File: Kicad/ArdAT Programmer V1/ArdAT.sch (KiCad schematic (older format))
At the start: 20 parts

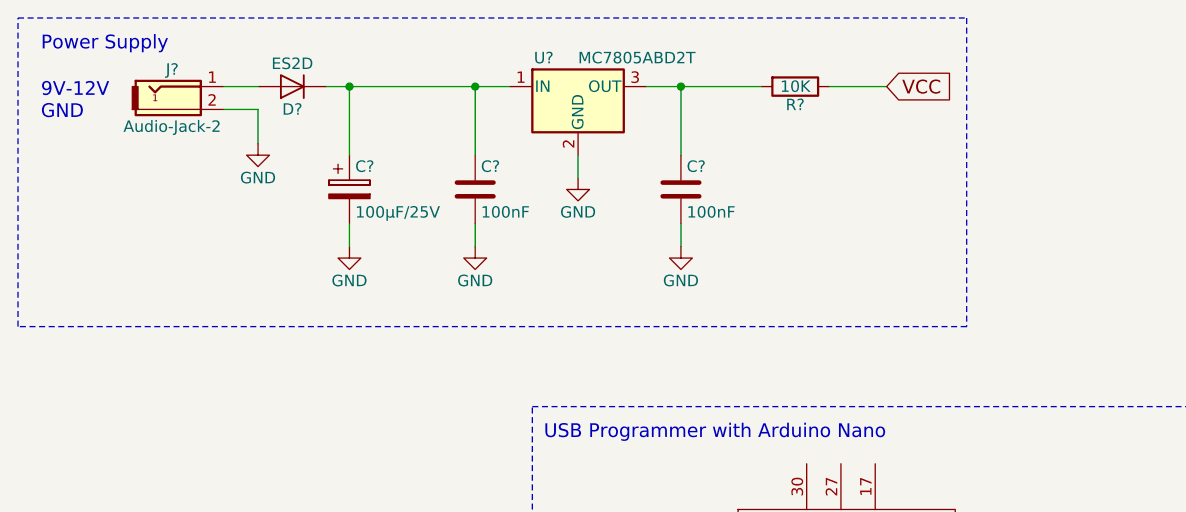
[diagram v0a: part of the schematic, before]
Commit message: Update
Update 3.3V
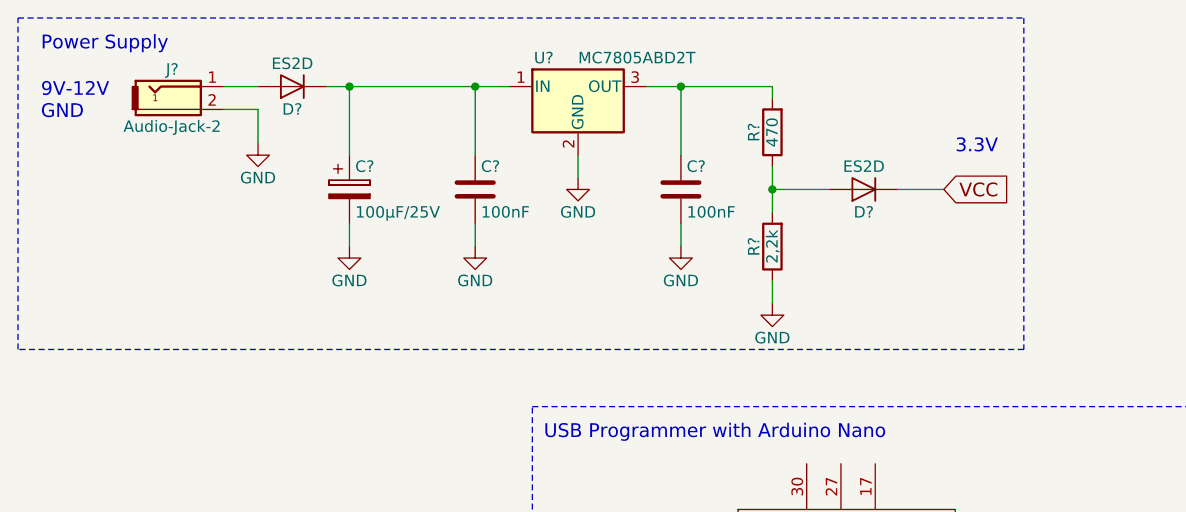
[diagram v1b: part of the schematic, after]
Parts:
- removed R?: 10K, symbol R
- added D?: ES2D, symbol D
- added R?: 470, symbol R
- added R?: 2,2k, symbol R
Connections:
- net GND: now also R?.1
- net VCC: now also D?.1 (K)
- net at C?.1, U?.3 (OUT): now also R?.2
- new net: D?.2 (A), R?.1, R?.2
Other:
- note added: "3.3V"
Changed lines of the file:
@@
 	1    0    0    -1
 $EndComp
-$Comp
-L R R?
-U 1 1 5AD70BC0
-P 4500 1000
-F 0 "R?" V 4580 1000 50  0000 C CNN
-F 1 "10K" V 4500 1000 50  0000 C CNN
-F 2 "" V 4430 1000 50  0001 C CNN
-F 3 "" H 4500 1000 50  0001 C CNN
-	1    4500 1000
-	0    1    1    0
-$EndComp
-Text GLabel 4900 1000 2    60   Input ~ 0
+Text GLabel 5150 1450 2    60   Input ~ 0
 VCC
 Text GLabel 8950 4000 0    60   Input ~ 0
@@
 F 3 "" H 2050 1000 50  0001 C CNN
 	1    1800 1000
-	1    0    0    -1
-$EndComp
-$Comp
-L MC7805ABD2T U?
-U 1 1 5AD7334E
-P 3550 1000
-F 0 "U?" H 3400 1125 50  0000 C CNN
-F 1 "MC7805ABD2T" H 3550 1125 50  0000 L CNN
-F 2 "" H 3575 850 50  0001 L CIN
-F 3 "" H 3550 950 50  0001 C CNN
-	1    3550 1000
 	1    0    0    -1
 $EndComp
@@
 	1550 6750 1550 5850
 Wire Wire Line
+	3100 1600 3100 1700
+Wire Wire Line
+	2550 1600 2550 1700
+Wire Wire Line
+	4000 1600 4000 1700
+Wire Wire Line
+	8950 3850 9400 3850
+Wire Wire Line
+	9400 3850 9400 3950
+Wire Wire Line
+	9400 3950 9500 3950
+Wire Wire Line
+	8950 4000 9350 4000
+Wire Wire Line
+	9350 4000 9350 4050
+Wire Wire Line
+	9350 4050 9500 4050
+Wire Wire Line
+	8950 4150 9500 4150
+Wire Wire Line
+	8950 4300 9350 4300
+Wire Wire Line
+	9350 4300 9350 4250
+Wire Wire Line
+	9350 4250 9500 4250
+Wire Wire Line
+	8950 4450 9400 4450
+Wire Wire Line
+	9400 4450 9400 4350
+Wire Wire Line
+	9400 4350 9500 4350
+Wire Wire Line
+	9500 4450 9450 4450
+Wire Wire Line
+	9450 4450 9450 4650
+Wire Wire Line
+	2000 1000 2150 1000
+Wire Wire Line
+	2000 1100 2150 1100
+Wire Wire Line
+	2150 1100 2150 1250
+Wire Notes Line
+	3350 2400 7300 2400
+Wire Notes Line
+	7300 2400 7300 6000
+Wire Notes Line
+	7300 6000 3350 6000
+Wire Notes Line
+	3350 6000 3350 2400
+Wire Notes Line
+	9150 5050 9450 5050
+Wire Notes Line
+	9450 5050 9450 5500
+Wire Notes Line
+	9450 5500 9150 5500
+Wire Notes Line
+	9150 5500 9150 5350
+Wire Notes Line
+	9100 5350 9450 5350
+Wire Notes Line
+	9100 5350 9100 5200
+Wire Notes Line
+	9100 5200 9450 5200
+Wire Notes Line
+	9150 5200 9150 5050
+Wire Notes Line
+	9300 5050 9300 5500
+Wire Notes Line
+	8550 3500 10350 3500
+Wire Notes Line
+	10350 3500 10350 5600
+Wire Notes Line
+	10350 5600 8550 5600
+Wire Notes Line
+	8550 5600 8550 3500
+$Comp
+L D D?
+U 1 1 5AD84211
+P 4800 1450
+F 0 "D?" H 4800 1550 50  0000 C CNN
+F 1 "ES2D" H 4800 1350 50  0000 C CNN
+F 2 "" H 4800 1450 50  0001 C CNN
+F 3 "" H 4800 1450 50  0001 C CNN
+	1    4800 1450
+	-1   0    0    1
+$EndComp
+Connection ~ 2550 1000
+Wire Wire Line
+	2550 1300 2550 1000
+Connection ~ 3100 1000
+Wire Wire Line
+	3100 1000 3100 1300
+Wire Wire Line
 	2450 1000 3250 1000
 Wire Wire Line
-	2550 1300 2550 1000
-Connection ~ 2550 1000
-Wire Wire Line
-	3100 1000 3100 1300
-Connection ~ 3100 1000
-Wire Wire Line
-	3850 1000 4350 1000
-Wire Wire Line
-	4000 1000 4000 1300
-Wire Wire Line
 	3550 1300 3550 1400
-Wire Wire Line
-	3100 1600 3100 1700
-Wire Wire Line
-	2550 1600 2550 1700
-Wire Wire Line
-	4000 1600 4000 1700
+$Comp
+L MC7805ABD2T U?
+U 1 1 5AD7334E
+P 3550 1000
+F 0 "U?" H 3400 1125 50  0000 C CNN
+F 1 "MC7805ABD2T" H 3550 1125 50  0000 L CNN
+F 2 "" H 3575 850 50  0001 L CIN
+F 3 "" H 3550 950 50  0001 C CNN
+	1    3550 1000
+	1    0    0    -1
+$EndComp
+$Comp
+L R R?
+U 1 1 5AD85C6A
+P 4400 1200
+F 0 "R?" V 4480 1200 50  0000 C CNN
+F 1 "470" V 4400 1200 50  0000 C CNN
+F 2 "" V 4330 1200 50  0001 C CNN
+F 3 "" H 4400 1200 50  0001 C CNN
+	1    4400 1200
+	-1   0    0    1
+$EndComp
+$Comp
+L R R?
+U 1 1 5AD85DF3
+P 4400 1700
+F 0 "R?" V 4480 1700 50  0000 C CNN
+F 1 "2,2k" V 4400 1700 50  0000 C CNN
+F 2 "" V 4330 1700 50  0001 C CNN
+F 3 "" H 4400 1700 50  0001 C CNN
+	1    4400 1700
+	-1   0    0    1
+$EndComp
+$Comp
+L GND #PWR?
+U 1 1 5AD85E4B
+P 4400 1950
+F 0 "#PWR?" H 4400 1700 50  0001 C CNN
+F 1 "GND" H 4400 1800 50  0000 C CNN
+F 2 "" H 4400 1950 50  0001 C CNN
+F 3 "" H 4400 1950 50  0001 C CNN
+	1    4400 1950
+	1    0    0    -1
+$EndComp
+Wire Wire Line
+	3850 1000 4400 1000
+Wire Wire Line
+	4400 1000 4400 1050
+Wire Wire Line
+	4400 1350 4400 1550
+Wire Wire Line
+	4650 1450 4400 1450
+Connection ~ 4400 1450
+Wire Wire Line
+	4000 1300 4000 1000
 Connection ~ 4000 1000
 Wire Wire Line
-	4650 1000 4900 1000
-Wire Wire Line
-	8950 3850 9400 3850
-Wire Wire Line
-	9400 3850 9400 3950
-Wire Wire Line
-	9400 3950 9500 3950
-Wire Wire Line
-	8950 4000 9350 4000
-Wire Wire Line
-	9350 4000 9350 4050
-Wire Wire Line
-	9350 4050 9500 4050
-Wire Wire Line
-	8950 4150 9500 4150
-Wire Wire Line
-	8950 4300 9350 4300
-Wire Wire Line
-	9350 4300 9350 4250
-Wire Wire Line
-	9350 4250 9500 4250
-Wire Wire Line
-	8950 4450 9400 4450
-Wire Wire Line
-	9400 4450 9400 4350
-Wire Wire Line
-	9400 4350 9500 4350
-Wire Wire Line
-	9500 4450 9450 4450
-Wire Wire Line
-	9450 4450 9450 4650
-Wire Wire Line
-	2000 1000 2150 1000
-Wire Wire Line
-	2000 1100 2150 1100
-Wire Wire Line
-	2150 1100 2150 1250
-Wire Notes Line
-	1100 700  5250 700
-Wire Notes Line
-	5250 700  5250 2050
-Wire Notes Line
-	5250 2050 1100 2050
-Wire Notes Line
-	1100 2050 1100 700
-Wire Notes Line
-	3350 2400 7300 2400
-Wire Notes Line
-	7300 2400 7300 6000
-Wire Notes Line
-	7300 6000 3350 6000
-Wire Notes Line
-	3350 6000 3350 2400
-Wire Notes Line
-	9150 5050 9450 5050
-Wire Notes Line
-	9450 5050 9450 5500
-Wire Notes Line
-	9450 5500 9150 5500
-Wire Notes Line
-	9150 5500 9150 5350
-Wire Notes Line
-	9100 5350 9450 5350
-Wire Notes Line
-	9100 5350 9100 5200
-Wire Notes Line
-	9100 5200 9450 5200
-Wire Notes Line
-	9150 5200 9150 5050
-Wire Notes Line
-	9300 5050 9300 5500
-Wire Notes Line
-	8550 3500 10350 3500
-Wire Notes Line
-	10350 3500 10350 5600
-Wire Notes Line
-	10350 5600 8550 5600
-Wire Notes Line
-	8550 5600 8550 3500
+	4400 1850 4400 1950
+Wire Wire Line
+	4950 1450 5150 1450
+Text Notes 5200 1300 0    60   ~ 0
+3.3V
+Wire Notes Line
+	1100 700  5500 700
+Wire Notes Line
+	5500 700  5500 2150
+Wire Notes Line
+	5500 2150 1100 2150
+Wire Notes Line
+	1100 2150 1100 700
 $EndSCHEMATC

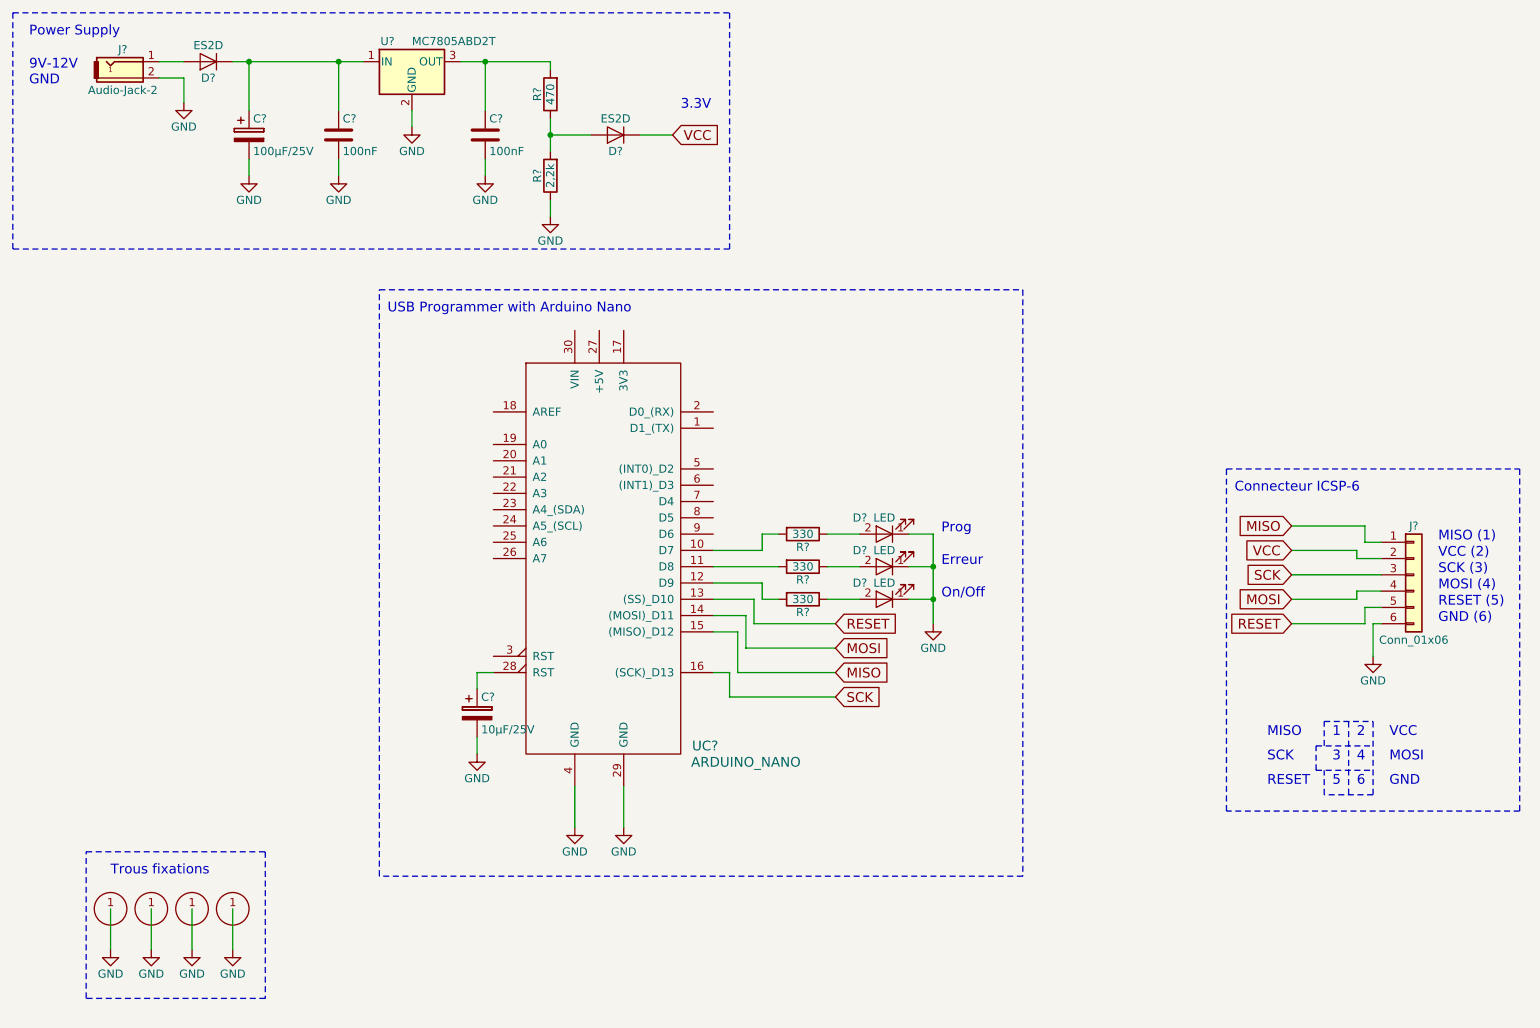
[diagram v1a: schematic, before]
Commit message: Create PCB
Create PCB
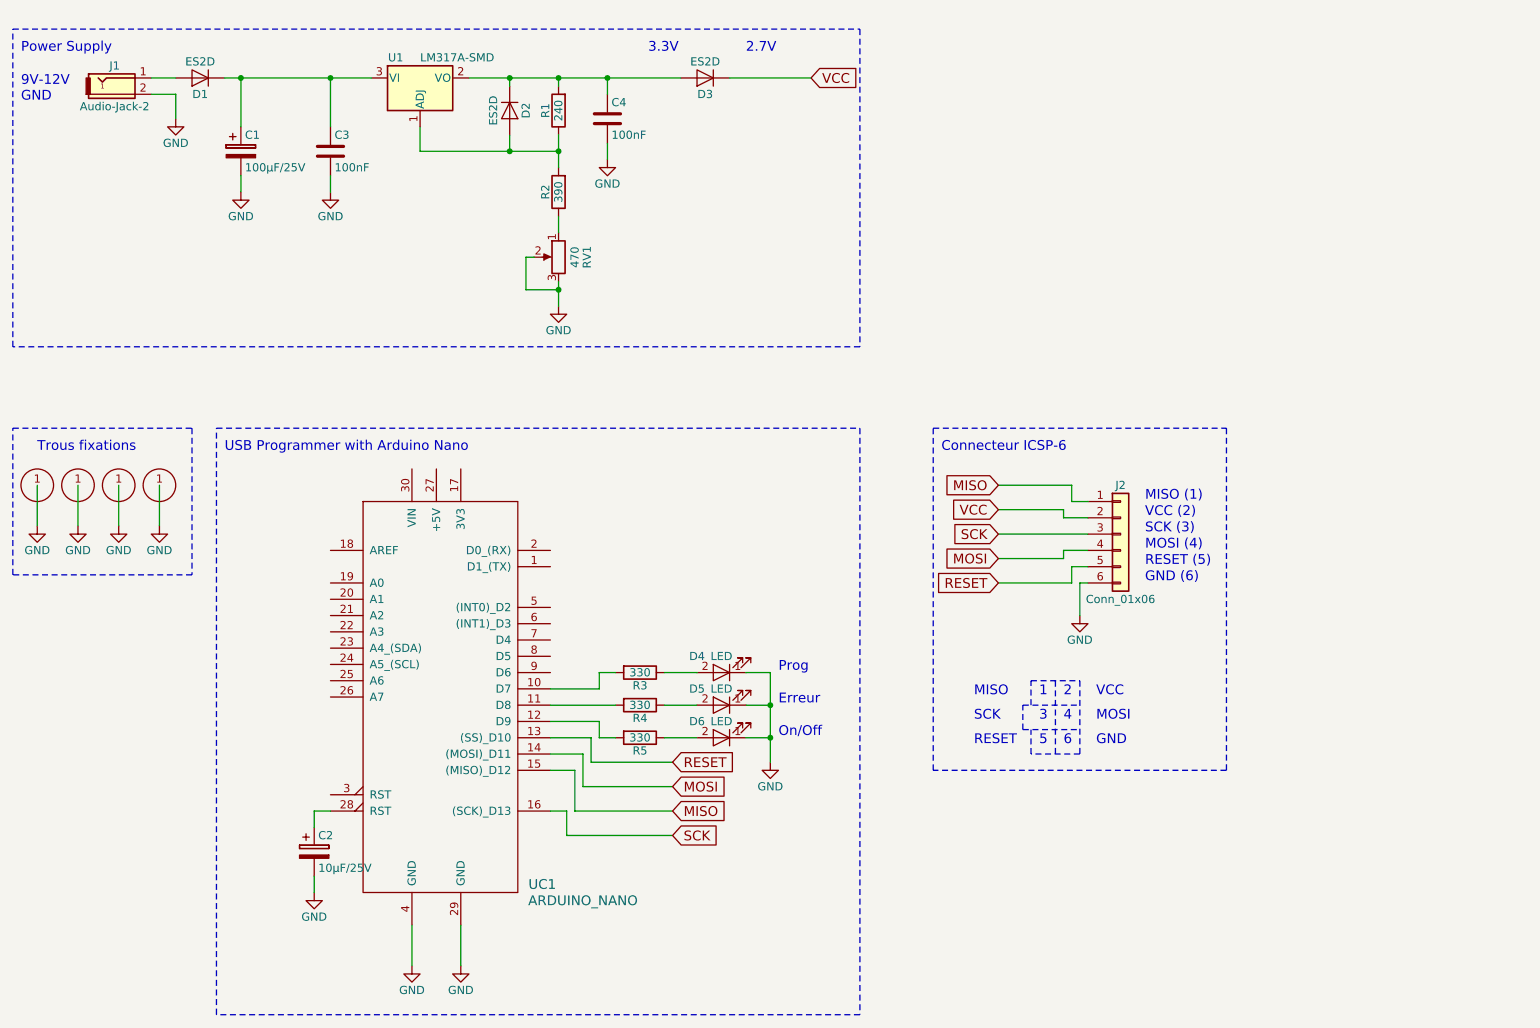
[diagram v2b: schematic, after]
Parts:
- removed U?: MC7805ABD2T, symbol MC7805ABD2T
- added D2: ES2D, alex-library:D0-214, symbol D
- added RV1: 470, alex-library:Potentiometer_Trimmer_Bourns_3296X, symbol POT
- added U1: LM317A-SMD, alex-library:T0-252-SMD, symbol LM317A-SMD
- C1: renamed from C?; footprint (none) -> alex-library:CP_Elec_6.3x7.7
- C2: renamed from C?; footprint (none) -> alex-library:CP_Elec_5x5.3
- C3, C4: renamed from C?; footprint (none) -> alex-library:C_0805_HandSoldering
- D1, D3: renamed from D?; footprint (none) -> alex-library:D0-214
- D4, D5, D6: renamed from D?; footprint (none) -> alex-library:LED_D3.0mm
- H1, H2, H3, H4: renamed from H?; footprint (none) -> alex-library:M3-Hole
- J1: renamed from J?; footprint (none) -> alex-library:Connect-2pin
- J2: renamed from J?; footprint (none) -> alex-library:2x3-Pin-Connecteur
- R1: renamed from R?; value 470 -> 240; footprint (none) -> alex-library:R_0805_HandSoldering
- R2: renamed from R?; value 2,2k -> 390; footprint (none) -> alex-library:R_0805_HandSoldering
- R3, R4, R5: renamed from R?; footprint (none) -> alex-library:R_0805_HandSoldering
- UC1: renamed from UC?; footprint (none) -> alex-library:ARDUINO_NANO
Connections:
- net GND: now also RV1.2, RV1.3; no longer R2.1
- net at C1.1, C3.1, D1.1 (K): now also U1.3 (VI)
- net at C4.1, R1.2: now also D3.2 (A), D2.1 (K), U1.2 (VO)
- net at R1.1, R2.2: now also D2.2 (A), U1.1 (ADJ); no longer D3.2 (A)
- new net: R2.1, RV1.1
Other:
- note added: "2.7V"
- moved on the sheet: C1, C2, C3, C4, D1, D3, D4, D5, D6, J1, J2, R1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

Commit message: Update
Update
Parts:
- J1: footprint alex-library:Connect-2pin -> alex-library:Connecteur-Embase-Debrochable-2_Voies
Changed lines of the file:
@@
 LIBS:valves
 LIBS:alex-library
-LIBS:ArdAT-cache
 EELAYER 25 0
 EELAYER END
@@
 F 0 "J1" H 1725 1175 50  0000 C CNN
 F 1 "Audio-Jack-2" H 1725 925 50  0000 C CNN
-F 2 "alex-library:Connect-2pin" H 2000 1100 50  0001 C CNN
+F 2 "alex-library:Connecteur-Embase-Debrochable-2_Voies" H 2000 1100 50  0001 C CNN
 F 3 "" H 2000 1100 50  0001 C CNN
 	1    1750 1100
